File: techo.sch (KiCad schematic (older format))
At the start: 194 parts, among them SW1 SW_Push, U1 ATmega32U4-AU, Y1 16MHz

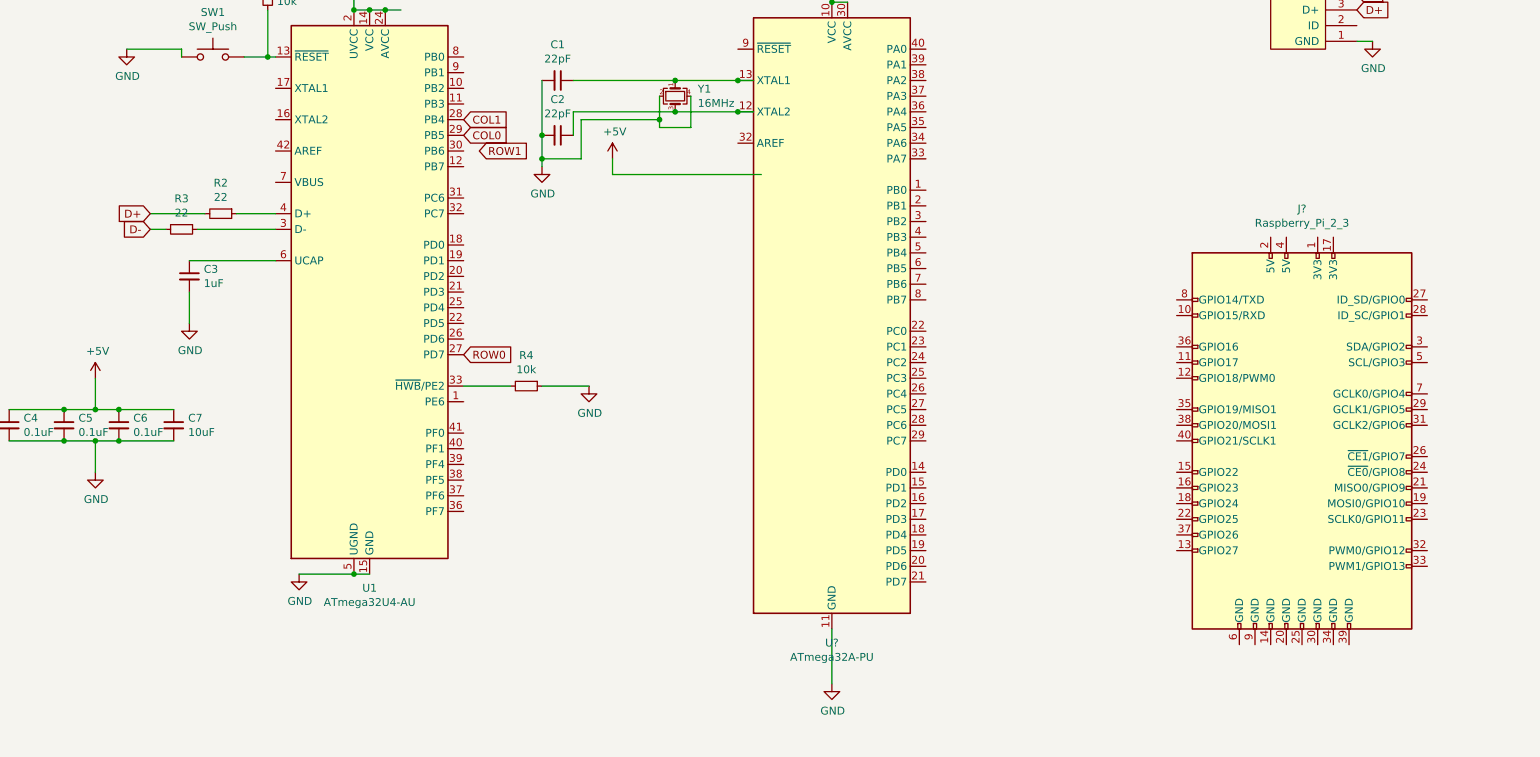
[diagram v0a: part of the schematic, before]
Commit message: Trying to do USB stuff
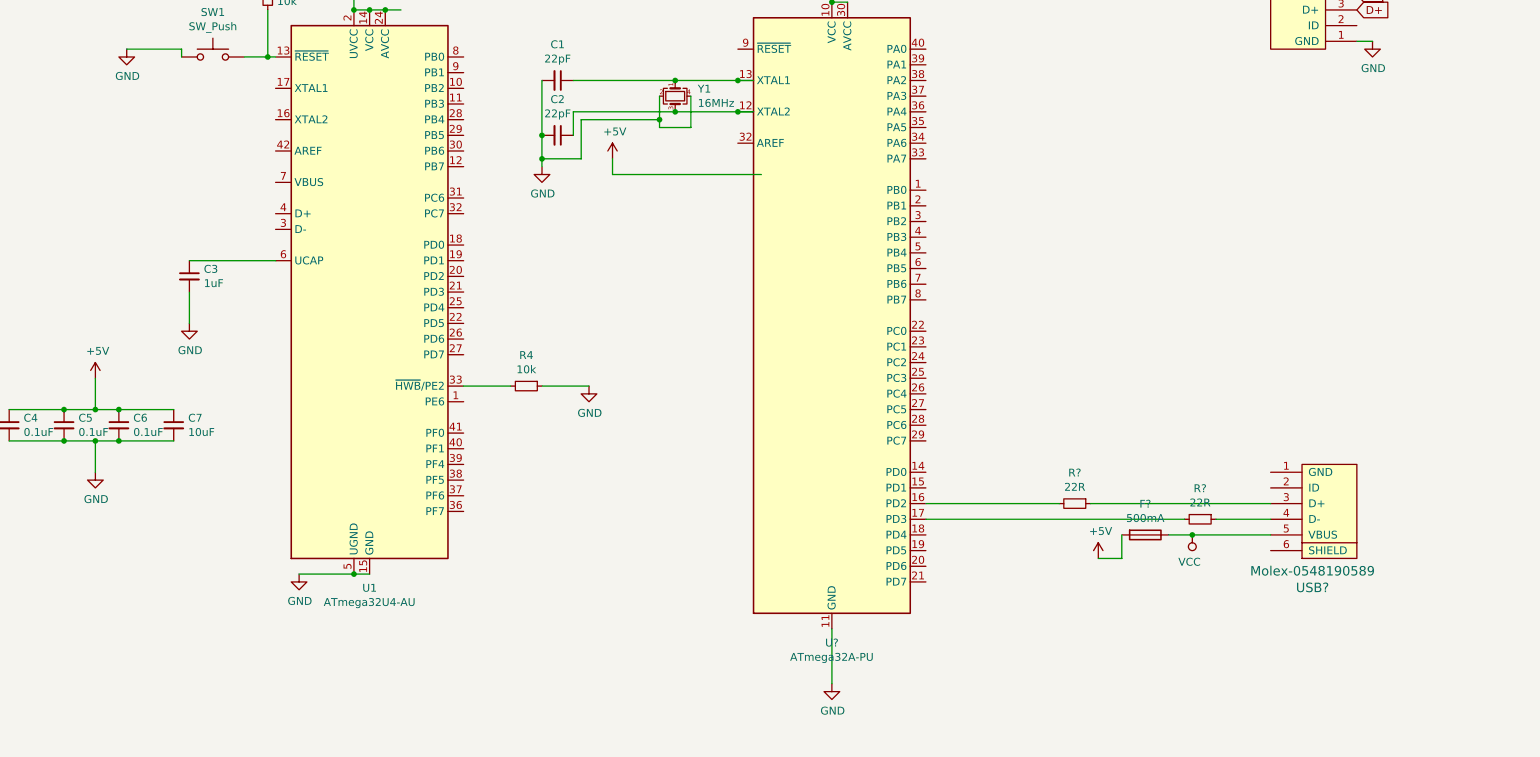
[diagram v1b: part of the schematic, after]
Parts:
- removed J?: Raspberry_Pi_2_3, symbol Connector:Raspberry_Pi_2_3
- removed R2, R3: 22, Resistor_SMD:R_0805_2012Metric, symbol Device:R_Small
- added F?: 500mA, symbol Device:Fuse
- added R? (x2): 22R, symbol Device:R_Small
- added USB?: Molex-0548190589, random-keyboard-parts:Molex-0548190589, symbol random-keyboard-parts:Molex-0548190589
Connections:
- wire segments 363 -> 367
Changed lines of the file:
@@
 	4000 3600 4300 3600
 $Comp
-L Device:R_Small R2
-U 1 1 6094A534
-P 1950 2500
-F 0 "R2" V 1754 2500 50  0000 C CNN
-F 1 "22" V 1845 2500 50  0000 C CNN
-F 2 "Resistor_SMD:R_0805_2012Metric" H 1950 2500 50  0001 C CNN
-F 3 "~" H 1950 2500 50  0001 C CNN
-	1    1950 2500
-	0    1    1    0
-$EndComp
-$Comp
-L Device:R_Small R3
-U 1 1 6094B389
-P 1700 2600
-F 0 "R3" V 1504 2600 50  0000 C CNN
-F 1 "22" V 1595 2600 50  0000 C CNN
-F 2 "Resistor_SMD:R_0805_2012Metric" H 1700 2600 50  0001 C CNN
-F 3 "~" H 1700 2600 50  0001 C CNN
-	1    1700 2600
-	0    1    1    0
-$EndComp
-Wire Wire Line
-	2300 2500 2050 2500
-Wire Wire Line
-	2300 2600 1800 2600
-Wire Wire Line
-	1500 2500 1850 2500
-Wire Wire Line
-	1600 2600 1500 2600
-$Comp
 L Device:C_Small C3
 U 1 1 6094E121
@@
 Wire Wire Line
 	2250 900  2250 1000
-Text GLabel 1500 2500 0    50   Input ~ 0
-D+
-Text GLabel 1500 2600 0    50   Input ~ 0
-D-
-$Comp
-L random-keyboard-parts:Molex-0548190589 USB1
-U 1 1 6097DBBA
-P 8900 1200
-F 0 "USB1" V 9437 1167 60  0000 C CNN
-F 1 "Molex-0548190589" V 9331 1167 60  0000 C CNN
-F 2 "random-keyboard-parts:Molex-0548190589" H 8900 1200 60  0001 C CNN
-F 3 "" H 8900 1200 60  0001 C CNN
-	1    8900 1200
-	0    -1   -1   0
-$EndComp
-$Comp
-L power:VCC #PWR0111
-U 1 1 6098043C
-P 9550 1000
-F 0 "#PWR0111" H 9550 850 50  0001 C CNN
-F 1 "VCC" H 9567 1173 50  0000 C CNN
-F 2 "" H 9550 1000 50  0001 C CNN
-F 3 "" H 9550 1000 50  0001 C CNN
-	1    9550 1000
-	1    0    0    -1
-$EndComp
-$Comp
-L Device:Polyfuse F1
-U 1 1 6098105B
-P 9950 1000
-F 0 "F1" V 9725 1000 50  0000 C CNN
-F 1 "500mA" V 9816 1000 50  0000 C CNN
-F 2 "Fuse:Fuse_1206_3216Metric" H 10000 800 50  0001 L CNN
-F 3 "~" H 9950 1000 50  0001 C CNN
-	1    9950 1000
-	0    1    1    0
-$EndComp
-$Comp
-L power:+5V #PWR0112
-U 1 1 60981543
-P 10350 1000
-F 0 "#PWR0112" H 10350 850 50  0001 C CNN
-F 1 "+5V" H 10365 1173 50  0000 C CNN
-F 2 "" H 10350 1000 50  0001 C CNN
-F 3 "" H 10350 1000 50  0001 C CNN
-	1    10350 1000
-	1    0    0    -1
-$EndComp
-Wire Wire Line
-	10100 1000 10350 1000
-Wire Wire Line
-	9550 1000 9800 1000
-Wire Wire Line
-	9550 1000 9200 1000
-Connection ~ 9550 1000
-Text GLabel 9200 1200 2    50   Input ~ 0
-D+
-Text GLabel 9200 1100 2    50   Input ~ 0
-D-
-$Comp
-L power:GND #PWR0113
-U 1 1 609872FD
-P 9300 1400
-F 0 "#PWR0113" H 9300 1150 50  0001 C CNN
-F 1 "GND" H 9305 1227 50  0000 C CNN
-F 2 "" H 9300 1400 50  0001 C CNN
-F 3 "" H 9300 1400 50  0001 C CNN
-	1    9300 1400
-	1    0    0    -1
-$EndComp
-Wire Wire Line
-	9200 1400 9300 1400
 $Comp
 L MX_Alps_Hybrid:MX-NoLED MX1
@@
 Wire Wire Line
 	7900 11400 7650 11400
-Text GLabel 3500 1900 2    50   Input ~ 0
-COL1
-Text GLabel 3500 2000 2    50   Input ~ 0
-COL0
-Text GLabel 3600 2100 2    50   Input ~ 0
-ROW1
-Text GLabel 3500 3400 2    50   Input ~ 0
-ROW0
 $Comp
 L MX_Alps_Hybrid:MX-NoLED MX14
@@
 Connection ~ 5250 1850
 Connection ~ 4850 1850
+Wire Wire Line
+	9200 1400 9300 1400
 $Comp
-L Connector:Raspberry_Pi_2_3 J?
-U 1 1 60969EEE
-P 8850 3950
-F 0 "J?" H 8850 5431 50  0000 C CNN
-F 1 "Raspberry_Pi_2_3" H 8850 5340 50  0000 C CNN
-F 2 "" H 8850 3950 50  0001 C CNN
-F 3 "https://www.raspberrypi.org/documentation/hardware/raspberrypi/schematics/rpi_SCH_3bplus_1p0_reduced.pdf" H 8850 3950 50  0001 C CNN
-	1    8850 3950
+L power:GND #PWR0113
+U 1 1 609872FD
+P 9300 1400
+F 0 "#PWR0113" H 9300 1150 50  0001 C CNN
+F 1 "GND" H 9305 1227 50  0000 C CNN
+F 2 "" H 9300 1400 50  0001 C CNN
+F 3 "" H 9300 1400 50  0001 C CNN
+	1    9300 1400
+	1    0    0    -1
+$EndComp
+Text GLabel 9200 1100 2    50   Input ~ 0
+D-
+Text GLabel 9200 1200 2    50   Input ~ 0
+D+
+Wire Wire Line
+	10100 1000 10350 1000
+$Comp
+L power:+5V #PWR0112
+U 1 1 60981543
+P 10350 1000
+F 0 "#PWR0112" H 10350 850 50  0001 C CNN
+F 1 "+5V" H 10365 1173 50  0000 C CNN
+F 2 "" H 10350 1000 50  0001 C CNN
+F 3 "" H 10350 1000 50  0001 C CNN
+	1    10350 1000
+	1    0    0    -1
+$EndComp
+$Comp
+L Device:Polyfuse F1
+U 1 1 6098105B
+P 9950 1000
+F 0 "F1" V 9725 1000 50  0000 C CNN
+F 1 "500mA" V 9816 1000 50  0000 C CNN
+F 2 "Fuse:Fuse_1206_3216Metric" H 10000 800 50  0001 L CNN
+F 3 "~" H 9950 1000 50  0001 C CNN
+	1    9950 1000
+	0    1    1    0
+$EndComp
+Wire Wire Line
+	9550 1000 9200 1000
+Wire Wire Line
+	9550 1000 9800 1000
+Connection ~ 9550 1000
+$Comp
+L power:VCC #PWR0111
+U 1 1 6098043C
+P 9550 1000
+F 0 "#PWR0111" H 9550 850 50  0001 C CNN
+F 1 "VCC" H 9567 1173 50  0000 C CNN
+F 2 "" H 9550 1000 50  0001 C CNN
+F 3 "" H 9550 1000 50  0001 C CNN
+	1    9550 1000
 	1    0    0    -1
 $EndComp
+$Comp
+L random-keyboard-parts:Molex-0548190589 USB1
+U 1 1 6097DBBA
+P 8900 1200
+F 0 "USB1" V 9437 1167 60  0000 C CNN
+F 1 "Molex-0548190589" V 9331 1167 60  0000 C CNN
+F 2 "random-keyboard-parts:Molex-0548190589" H 8900 1200 60  0001 C CNN
+F 3 "" H 8900 1200 60  0001 C CNN
+	1    8900 1200
+	0    -1   -1   0
+$EndComp
+$Comp
+L random-keyboard-parts:Molex-0548190589 USB?
+U 1 1 60C89F17
+P 8950 4350
+F 0 "USB?" V 9487 4317 60  0000 C CNN
+F 1 "Molex-0548190589" V 9381 4317 60  0000 C CNN
+F 2 "random-keyboard-parts:Molex-0548190589" H 8950 4350 60  0001 C CNN
+F 3 "" H 8950 4350 60  0001 C CNN
+	1    8950 4350
+	0    1    1    0
+$EndComp
+$Comp
+L power:VCC #PWR?
+U 1 1 60CD4FC7
+P 8150 4550
+F 0 "#PWR?" H 8150 4400 50  0001 C CNN
+F 1 "VCC" H 8168 4723 50  0000 C CNN
+F 2 "" H 8150 4550 50  0001 C CNN
+F 3 "" H 8150 4550 50  0001 C CNN
+	1    8150 4550
+	-1   0    0    1
+$EndComp
+Wire Wire Line
+	8650 4550 8150 4550
+$Comp
+L Device:Fuse F?
+U 1 1 60CFD39F
+P 7850 4550
+F 0 "F?" V 7653 4550 50  0000 C CNN
+F 1 "500mA" V 7744 4550 50  0000 C CNN
+F 2 "" V 7780 4550 50  0001 C CNN
+F 3 "~" H 7850 4550 50  0001 C CNN
+	1    7850 4550
+	0    1    1    0
+$EndComp
+Wire Wire Line
+	8150 4550 8000 4550
+Connection ~ 8150 4550
+$Comp
+L power:+5V #PWR?
+U 1 1 60D27519
+P 7550 4700
+F 0 "#PWR?" H 7550 4550 50  0001 C CNN
+F 1 "+5V" H 7565 4873 50  0000 C CNN
+F 2 "" H 7550 4700 50  0001 C CNN
+F 3 "" H 7550 4700 50  0001 C CNN
+	1    7550 4700
+	1    0    0    -1
+$EndComp
+Wire Wire Line
+	7700 4550 7700 4700
+Wire Wire Line
+	7700 4700 7550 4700
+Wire Wire Line
+	8650 4350 7500 4350
+Wire Wire Line
+	8650 4450 8300 4450
+$Comp
+L Device:R_Small R?
+U 1 1 60D9973F
+P 7400 4350
+F 0 "R?" V 7204 4350 50  0000 C CNN
+F 1 "22R" V 7295 4350 50  0000 C CNN
+F 2 "" H 7400 4350 50  0001 C CNN
+F 3 "~" H 7400 4350 50  0001 C CNN
+	1    7400 4350
+	0    1    1    0
+$EndComp
+Wire Wire Line
+	7300 4350 6450 4350
+$Comp
+L Device:R_Small R?
+U 1 1 60D9AF2B
+P 8200 4450
+F 0 "R?" V 8004 4450 50  0000 C CNN
+F 1 "22R" V 8095 4450 50  0000 C CNN
+F 2 "" H 8200 4450 50  0001 C CNN
+F 3 "~" H 8200 4450 50  0001 C CNN
+	1    8200 4450
+	0    1    1    0
+$EndComp
+Wire Wire Line
+	8100 4450 6450 4450
 $EndSCHEMATC
